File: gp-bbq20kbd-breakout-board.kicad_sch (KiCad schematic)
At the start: 27 parts, among them J1 Power, J2 Keyboard, J3 Motion, J4 Mic, J5 Backlight, J6 Pico Board, J7 UART Pico, U1 TPS7A2033PDBVR, U2 TPS7A2018PDBVR, U3 TPS7A2028PDBVR

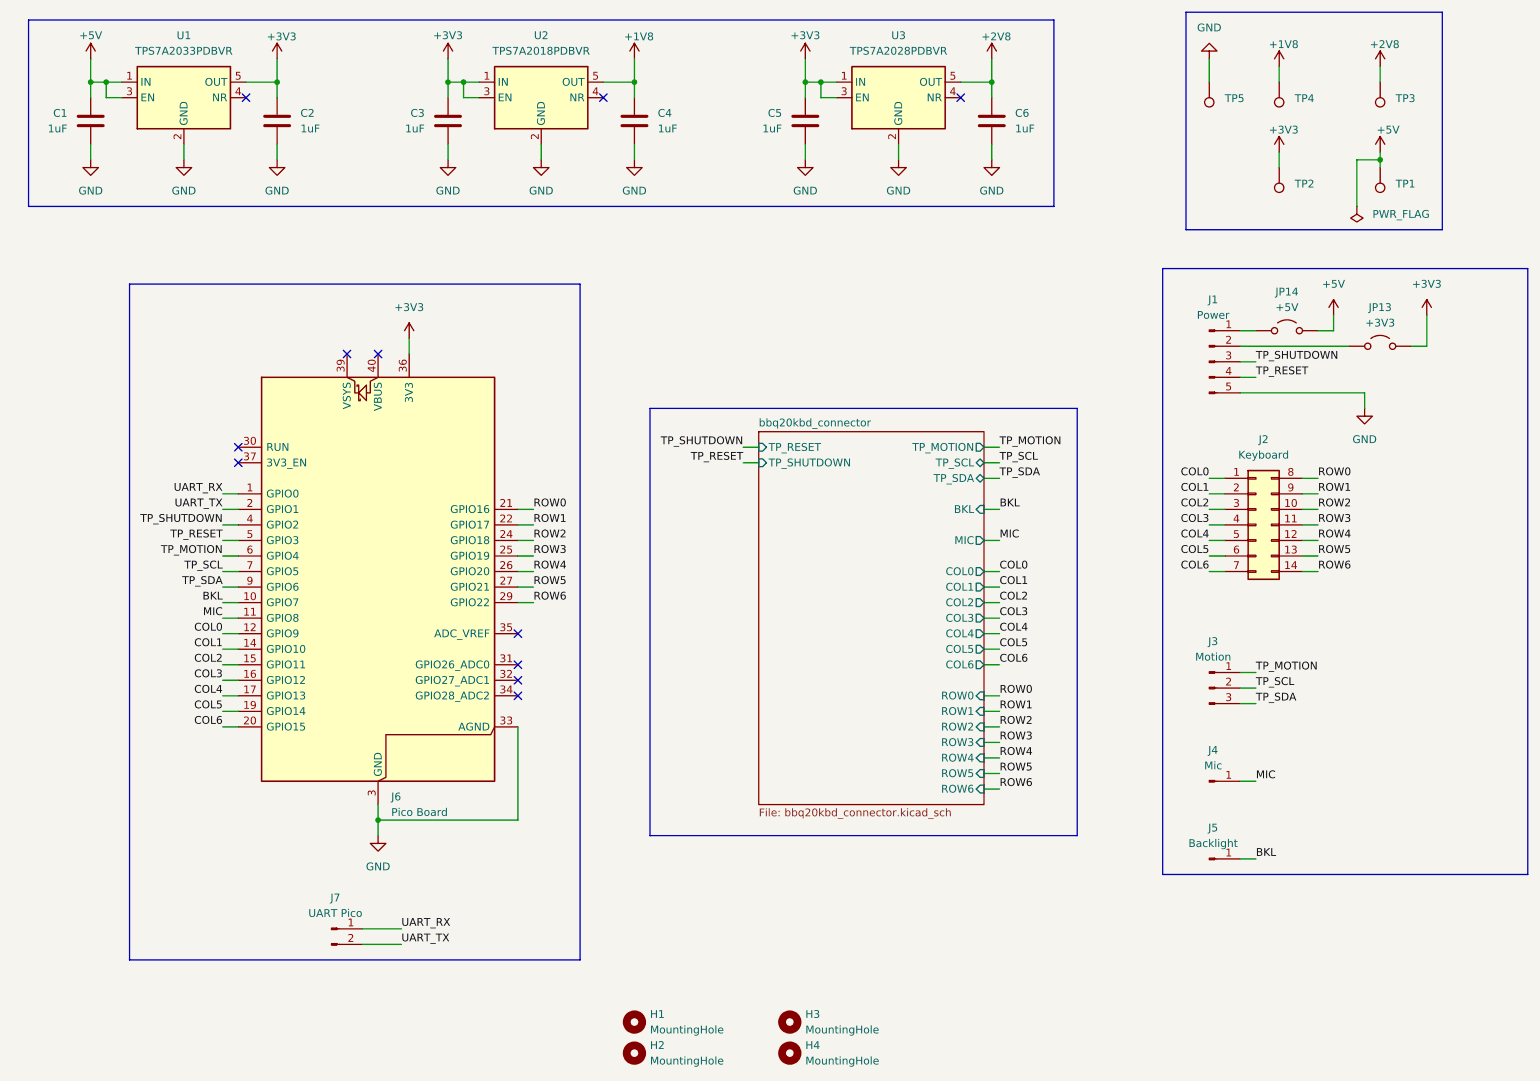
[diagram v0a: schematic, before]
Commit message: Begin PCB
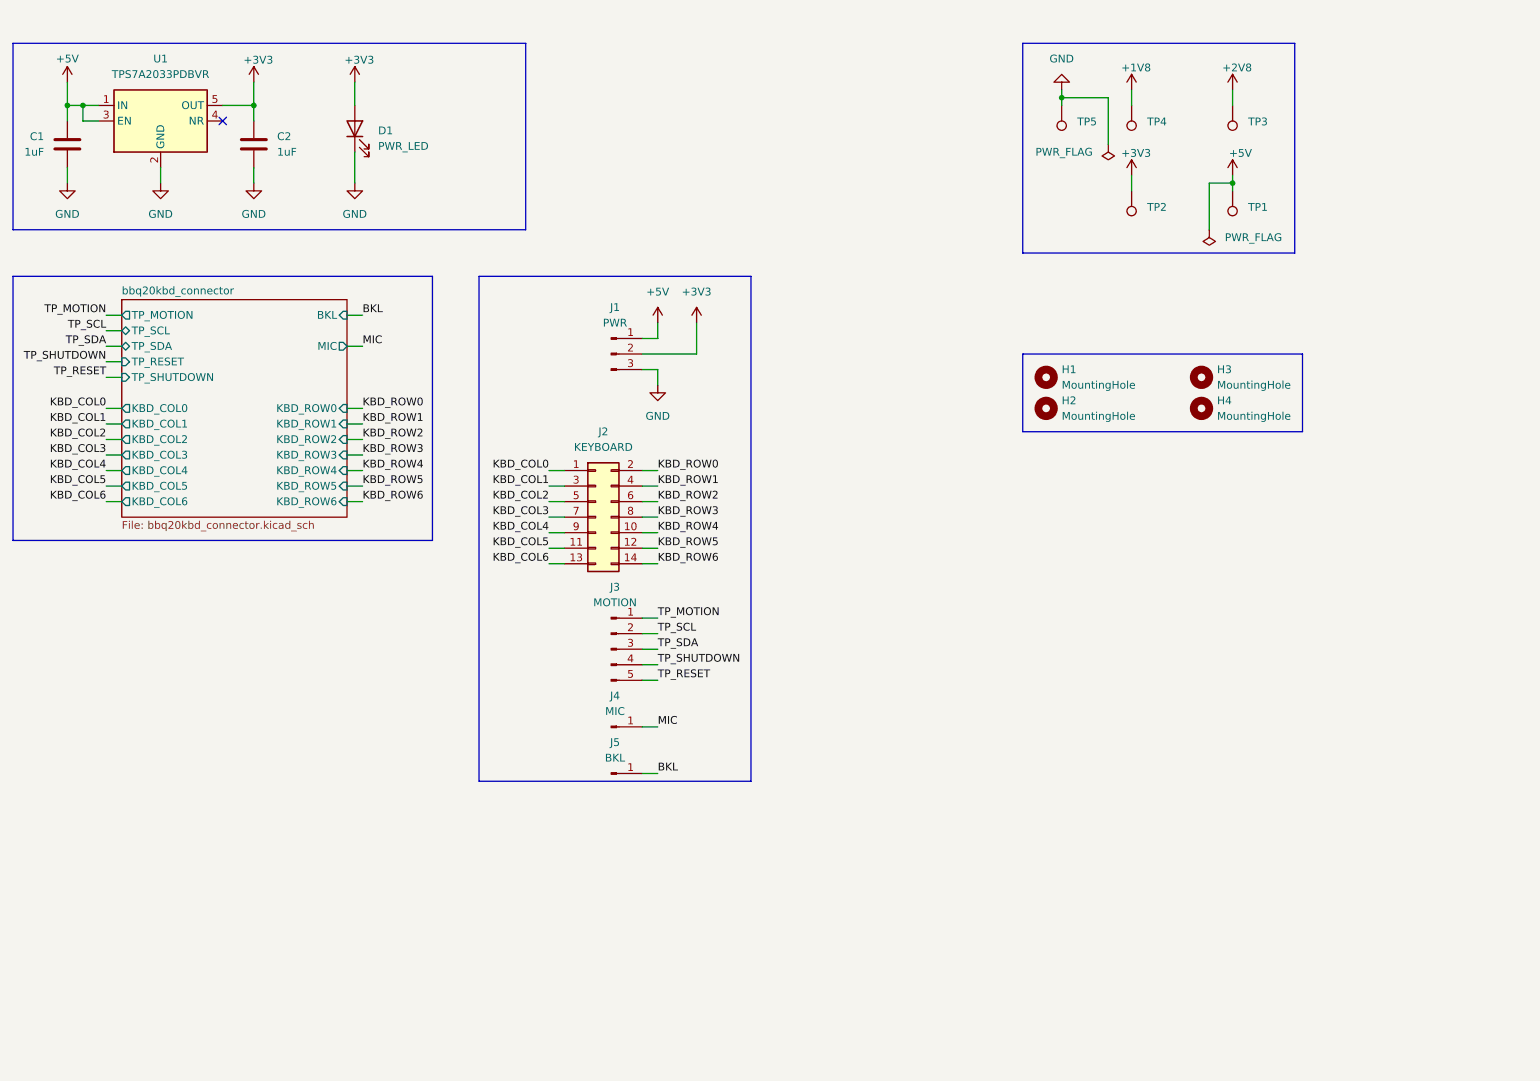
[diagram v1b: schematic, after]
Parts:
- removed C3, C4, C5, C6: 1uF, Capacitor_SMD:C_0603_1608Metric, symbol Device:C
- removed J6: Pico Board, Module:RaspberryPi_Pico_Common_THT, symbol MCU_Module:RaspberryPi_Pico
- removed J7: UART Pico, Connector_PinHeader_2.54mm:PinHeader_1x02_P2.54mm_Vertical, symbol Connector:Conn_01x02_Pin
- removed JP13: +3V3, TestPoint:TestPoint_2Pads_Pitch2.54mm_Drill0.8mm, symbol Jumper:Jumper_2_Open
- removed JP14: +5V, TestPoint:TestPoint_2Pads_Pitch2.54mm_Drill0.8mm, symbol Jumper:Jumper_2_Open
- removed U2: TPS7A2018PDBVR, Package_TO_SOT_SMD:SOT-23-5, symbol Regulator_Linear:TPS73618DBV
- removed U3: TPS7A2028PDBVR, Package_TO_SOT_SMD:SOT-23-5, symbol Regulator_Linear:TPS73618DBV
- added D1: PWR_LED, LED_SMD:LED_0603_1608Metric, symbol Device:LED
- J1: renamed from J3; value Motion -> PWR
- J2: value Keyboard -> KEYBOARD; symbol Connector_Generic:Conn_02x07_Top_Bottom -> Connector_Generic:Conn_02x07_Odd_Even
- J3: renamed from J1; value Power -> MOTION; footprint Connector_PinSocket_2.54mm:PinSocket_1x05_P2.54mm_Vertical -> Connector_PinHeader_2.54mm:PinHeader_1x05_P2.54mm_Vertical
- J4: value Mic -> MIC
- J5: value Backlight -> BKL
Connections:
- net +3V3: now also J1.2 (Pin_2), D1.2 (A)
- net +5V: now also J1.1 (Pin_1)
- net GND: now also J1.3 (Pin_3), D1.1 (K); no longer J3.5 (Pin_5)
- net TP_MOTION: now also J3.1 (Pin_1); no longer J1.1 (Pin_1)
- net TP_RESET: now also J3.5 (Pin_5); no longer J3.4 (Pin_4)
- net TP_SCL: now also J3.2 (Pin_2); no longer J1.2 (Pin_2)
- net TP_SDA: now also J3.3 (Pin_3); no longer J1.3 (Pin_3)
- net TP_SHUTDOWN: now also J3.4 (Pin_4); no longer J3.3 (Pin_3)
- net COL0 renamed KBD_COL0
- net COL1 renamed KBD_ROW0
- net COL2 renamed KBD_COL1
- net COL3 renamed KBD_ROW1
- net COL4 renamed KBD_COL2
- net COL5 renamed KBD_ROW2
- net COL6 renamed KBD_COL3
- net ROW0 renamed KBD_ROW3
- net ROW1 renamed KBD_COL4
- net ROW2 renamed KBD_ROW4
- net ROW3 renamed KBD_COL5
- net ROW4 renamed KBD_ROW5
- net ROW5 renamed KBD_COL6
- net ROW6 renamed KBD_ROW6
- no-connect marks 11 -> 1
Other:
- sheet bbq20kbd_connector ports: added KBD_COL0, KBD_COL1, KBD_COL2, KBD_COL3, KBD_COL4, KBD_COL5, KBD_COL6, KBD_ROW0, KBD_ROW1, KBD_ROW2, KBD_ROW3, KBD_ROW4, KBD_ROW5, KBD_ROW6; removed COL0, COL1, COL2, COL3, COL4, COL5, COL6, ROW0, ROW1, ROW2, ROW3, ROW4, ROW5, ROW6
- moved on the sheet: C1, C2, H1, H2, H3, H4, J1, J2, J3, J4, J5, TP1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
